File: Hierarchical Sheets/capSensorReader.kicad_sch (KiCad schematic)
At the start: 13 parts, among them U2 LM358, U3 LM358

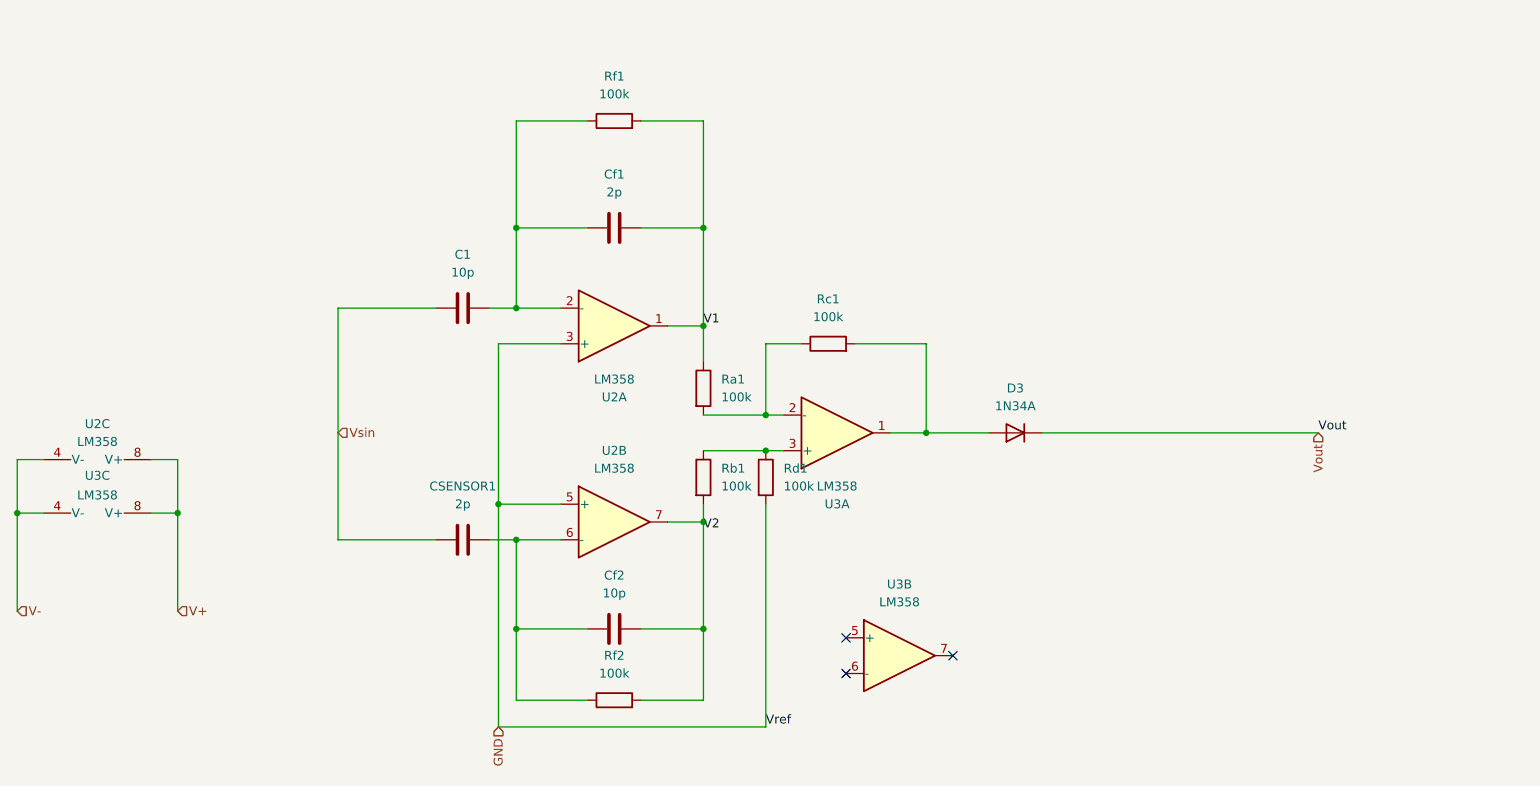
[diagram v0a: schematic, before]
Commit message: Update Main Sub Sheets
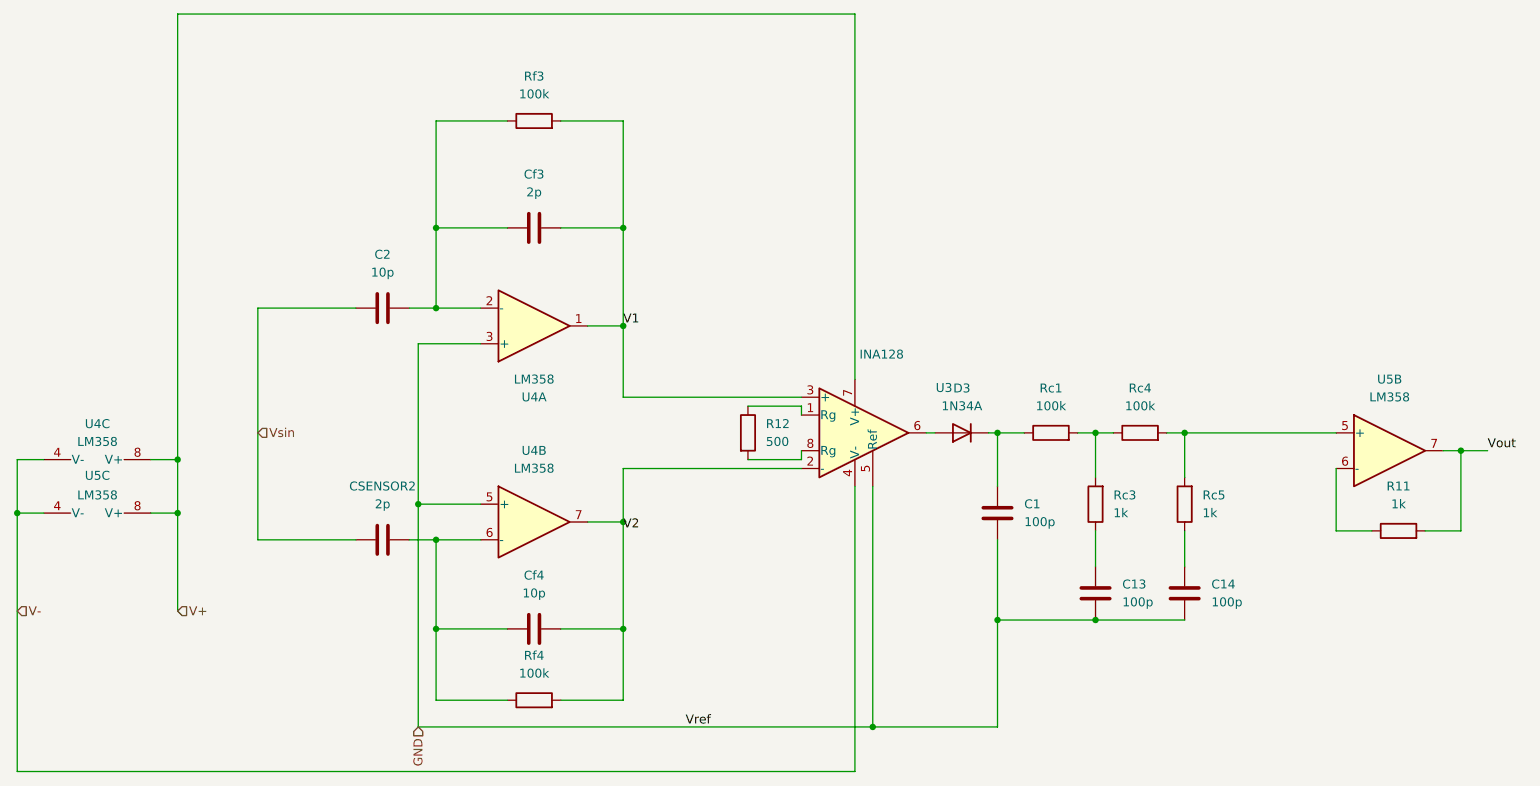
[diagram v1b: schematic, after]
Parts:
- removed Ra1, Rb1, Rd1: 100k, Resistor_THT:R_Axial_DIN0204_L3.6mm_D1.6mm_P5.08mm_Horizontal, symbol Device:R
- removed unit 1 of U3
- added C1, C13, C14: 100p, symbol Device:C
- added R11, Rc3, Rc5: 1k, symbol Device:R
- added R12: 500, symbol Device:R
- added Rc4: 100k, symbol Device:R
- added U3: INA128, symbol Amplifier_Instrumentation:INA128
- Rc1: footprint Resistor_THT:R_Axial_DIN0204_L3.6mm_D1.6mm_P5.08mm_Horizontal -> (none)
- renumbered C1 to C2, CSENSOR1 to CSENSOR2, Cf1 to Cf3, Cf2 to Cf4, Rf1 to Rf3, Rf2 to Rf4, U2 to U4, U3 to U5
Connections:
- net GND: now also C1.2, C13.2, C14.2, U3.5 (Ref)
- net V+: now also U3.7 (V+)
- net V-: now also U3.4 (V-)
- net V1: now also U3.3 (+)
- net V2: now also U3.2 (-)
- net Vout: now also U5.7, R11.2; no longer D3.1 (K)
- net at Rc1.1: now also D3.1 (K), C1.1
- net at Rc1.2: now also Rc3.2, Rc4.1; no longer D3.2 (A)
- net at U5.5 (+): now also Rc4.2, Rc5.2
- net at U5.6 (-): now also R11.1
- new net: C14.1, Rc5.1
- new net: R12.1, U3.1 (Rg)
- new net: D3.2 (A), U3.6
- new net: R12.2, U3.8 (Rg)
- new net: C13.1, Rc3.1
- no-connect marks 3 -> 0
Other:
- moved on the sheet: C2, CSENSOR2, Cf3, Cf4, Rf3, Rf4, U4A, U4B, U5B
